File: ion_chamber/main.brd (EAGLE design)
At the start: 7 parts, among them Q1 SST201

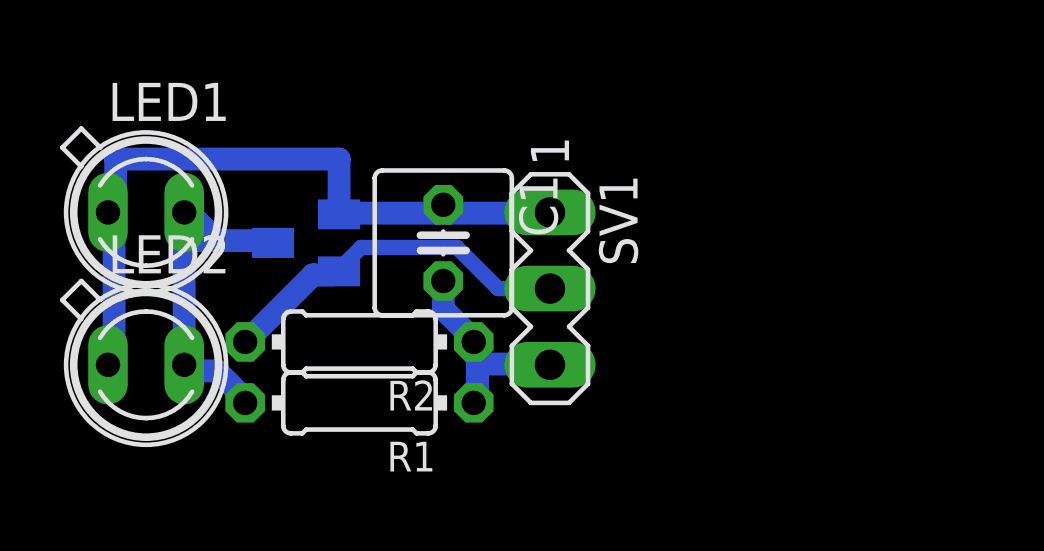
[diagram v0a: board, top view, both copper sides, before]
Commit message: Output files added.
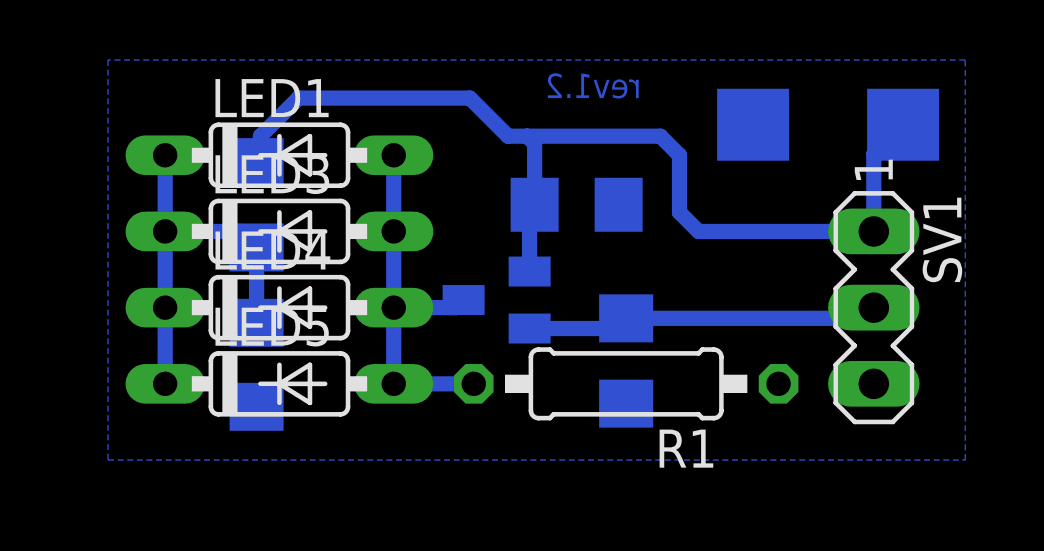
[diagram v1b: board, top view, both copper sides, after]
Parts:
- removed LED2: (no value), led:SFH480
- added C2: 100n, resistor:C1206
- added C3: 100u, resistor:SMC_C
- added LED3, LED4, LED5: 1N4148, diode:DO35-7
- added R3: 100k, resistor:R1206
- C1: value (none) -> 100n; device resistor:C025-050X050 -> resistor:C1206
- LED1: value (none) -> 1N4148; device led:SFH480 -> diode:DO35-7
- Q1: value SST201 -> J111
- R1: value (none) -> 10M; device resistor:0204/7 -> resistor:0207/10
- R2: value (none) -> 1k; device resistor:0204/7 -> resistor:R1206
- SV1: value (none) -> connector
- moved SV1 10.8 mm to (28.1, 56.5)
- moved R1 8.91 mm to (19.8, 54.0)
- moved C1 7.43 mm to (7.49, 54.6), flipped to the bottom
- moved Q1 6.63 mm to (15.5, 56.8)
- moved R2 5.72 mm to (7.49, 59.9), flipped to the bottom, turned to 270 degrees
- moved LED1 4.84 mm to (8.26, 61.6)
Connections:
- removed net N$3: C1.2, R1.1, R2.1, SV1.3
- new net GND: C1.2, C2.2, C3.-, R1.1, R3.1, SV1.3
- new net N$1: C1.1, LED1.C, LED3.C, LED4.C, LED5.C, R2.2
- net N$2: now also R3.2; no longer R2.2
- net N$4: now also LED3.A, LED4.A, LED5.A; no longer LED2.A
- net N$6: now also C2.1, C3.+, R2.1; no longer C1.1, LED1.K, LED2.K
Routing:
- net N$1: track 0.00 -> 13.4 mm
- net N$6: track 24.2 -> 33.5 mm
- net N$3: track 7.02 -> 0.00 mm
- net N$4: track 11.3 -> 12.7 mm
- added copper zone on layer 16, net GND
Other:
- board text added: "rev1.2"
